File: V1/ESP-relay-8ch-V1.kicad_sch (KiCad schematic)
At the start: 142 parts, among them J1 +24VDC, J10 OUT1, J2 INPUTS, J3 OUT1, J4 OUT1, J5 OUT1, J6 OUT1, J7 OUT1, J8 OUT1, J9 OUT1, K1 G5PZ-1A, K2 G5PZ-1A, K3 G5PZ-1A, K4 G5PZ-1A, K5 G5PZ-1A, K6 G5PZ-1A, K7 G5PZ-1A, K8 G5PZ-1A, Q1 MMBT2222A/SOT-23-3, Q2 MMBT2222A/SOT-23-3, Q3 MMBT2222A/SOT-23-3, Q4 MMBT2222A/SOT-23-3, Q5 MMBT2222A/SOT-23-3, Q6 MMBT2222A/SOT-23-3, Q7 MMBT2222A/SOT-23-3, Q8 MMBT2222A/SOT-23-3, U1 SY8089A1AAC, U10 TX4138, U11 Olimex_ESP32-POE, U2 LTV-817S, U3 LTV-817S, U4 LTV-817S, U5 LTV-817S, U6 LTV-817S, U7 LTV-817S, U8 LTV-817S, U9 LTV-817S

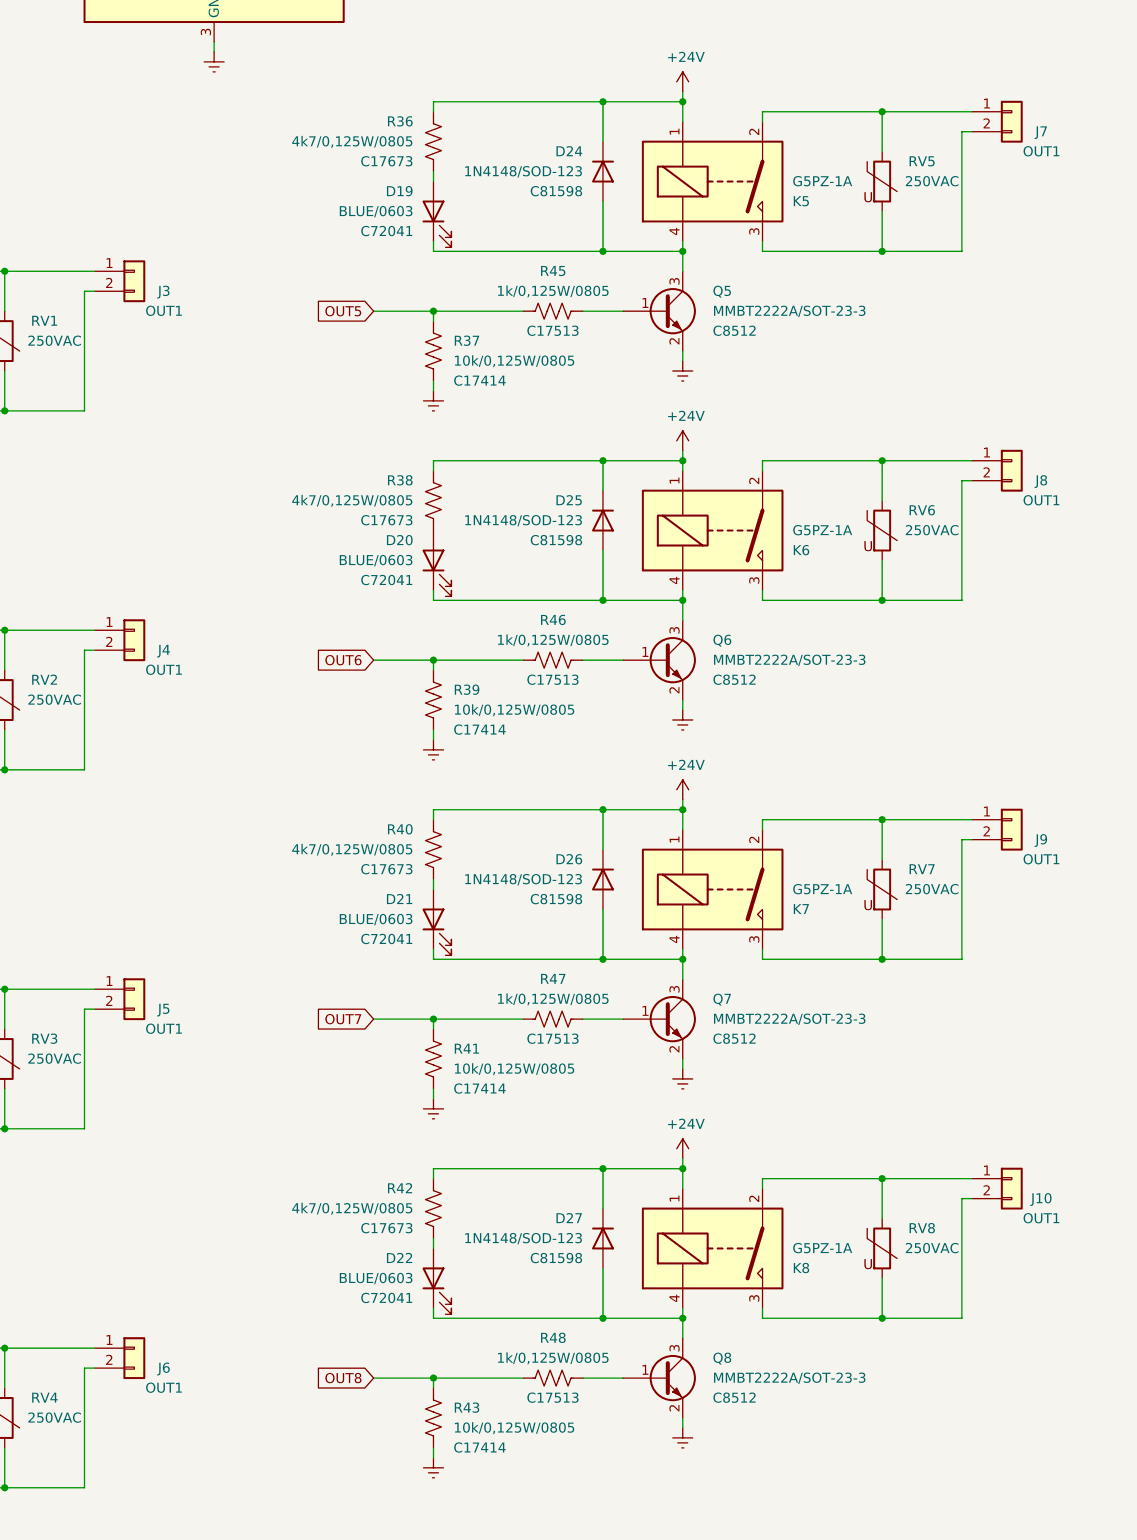
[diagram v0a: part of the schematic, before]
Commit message: Development
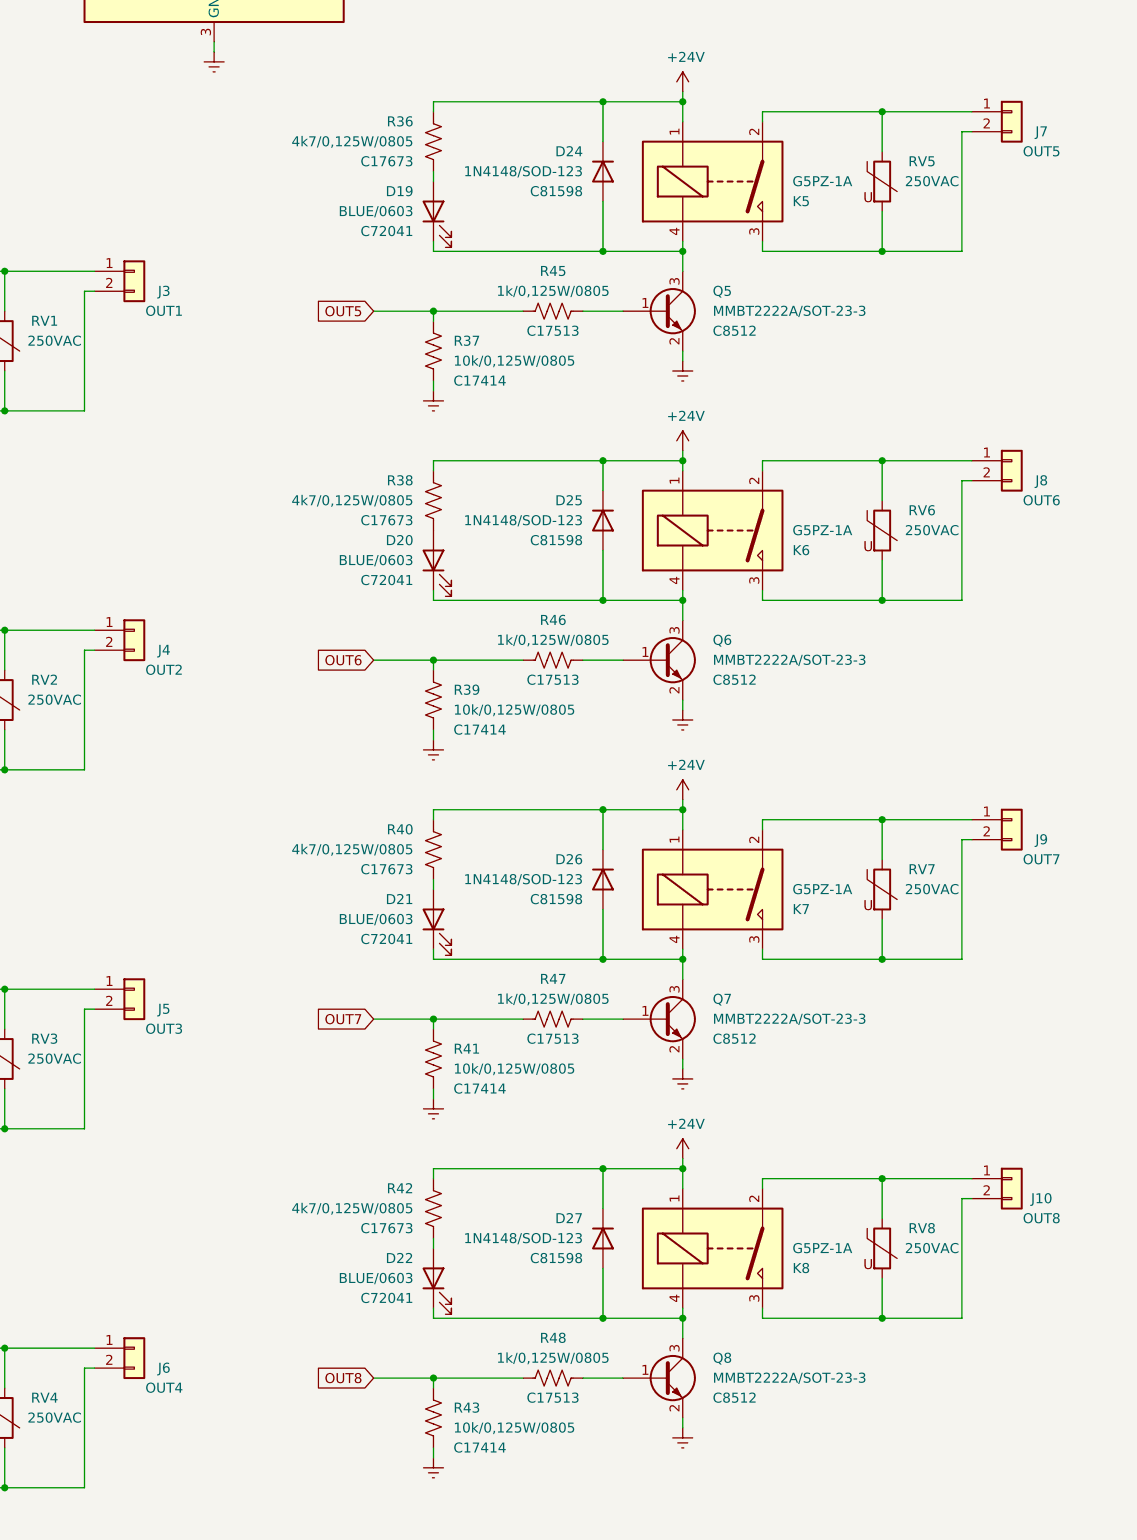
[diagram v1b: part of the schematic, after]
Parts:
- C1, C13: LCSC Part C1849 -> (none); LCSC Part # (none) -> C1849
- C10, C3, C4, C5, C6, C7, C8, C9: LCSC Part C1739 -> (none); LCSC Part # (none) -> C1739
- C11, C14: LCSC Part C49678 -> (none); LCSC Part # (none) -> C49678
- C12: LCSC Part C1653 -> (none); LCSC Part # (none) -> C1653
- C15: LCSC Part C38523 -> (none); LCSC Part # (none) -> C38523
- C16: LCSC Part C249930 -> (none); LCSC Part # (none) -> C249930
- C2: LCSC Part C263963 -> (none); LCSC Part # (none) -> C263963
- D1: LCSC Part C64898 -> (none); LCSC Part # (none) -> C64898
- D10: LCSC Part C65010 -> (none); LCSC Part # (none) -> C65010
- D11, D12, D13, D14, D19, D20, D21, D22: LCSC Part C72041 -> (none); LCSC Part # (none) -> C72041
- D15, D16, D17, D18, D24, D25, D26, D27: LCSC Part C81598 -> (none); LCSC Part # (none) -> C81598
- D2, D3, D4, D5, D6, D7, D8, D9: LCSC Part C109072 -> (none); LCSC Part # (none) -> C109072
- D23, D28, D29: LCSC Part C72043 -> (none); LCSC Part # (none) -> C72043
- J1: JLCPCB BOM (none) -> 0; Mfr (none) -> Metaltex; Mfr PN (none) -> BR902V; Vendor (none) -> Eletropeças; Vendor PN (none) -> 29273
- J10: value OUT1 -> OUT8
- J4: value OUT1 -> OUT2
- J5: value OUT1 -> OUT3
- J6: value OUT1 -> OUT4
- J7: value OUT1 -> OUT5
- J8: value OUT1 -> OUT6
- J9: value OUT1 -> OUT7
- L1: LCSC Part C370424 -> (none); LCSC Part # (none) -> C370424
- L2: LCSC Part C127788 -> (none); LCSC Part # (none) -> C127788
- Q1, Q2, Q3, Q4, Q5, Q6, Q7, Q8: LCSC Part C8512 -> (none); LCSC Part # (none) -> C8512
- R1, R2, R3, R4, R5, R6, R7, R8: LCSC Part C17379 -> (none); LCSC Part # (none) -> C17379
- R10: LCSC Part C149504 -> (none); LCSC Part # (none) -> C149504
- R11: LCSC Part C17552 -> (none); LCSC Part # (none) -> C17552
- R12, R13, R14, R15, R16, R17, R18, R19: LCSC Part C26010 -> (none); LCSC Part # (none) -> C26010
- R20: LCSC Part C17724 -> (none); LCSC Part # (none) -> C17724
- R21, R23, R25, R27, R35, R36, R38, R40, R42: LCSC Part C17673 -> (none); LCSC Part # (none) -> C17673
- R22, R24, R26, R28, R37, R39, R41, R43: LCSC Part C17414 -> (none); LCSC Part # (none) -> C17414
- R29: LCSC Part C17616 -> (none); LCSC Part # (none) -> C17616
- R30: LCSC Part C17758 -> (none); LCSC Part # (none) -> C17758
- R31, R32, R33, R34, R45, R46, R47, R48: LCSC Part C17513 -> (none); LCSC Part # (none) -> C17513
- R44: LCSC Part C4382 -> (none); LCSC Part # (none) -> C4382
- R49: LCSC Part C17837 -> (none); LCSC Part # (none) -> C17837
- R50: LCSC Part C17630 -> (none); LCSC Part # (none) -> C17630
- R9: LCSC Part C247605 -> (none); LCSC Part # (none) -> C247605
- U1: LCSC Part C479074 -> (none); LCSC Part # (none) -> C479074
- U10: LCSC Part C329267 -> (none); LCSC Part # (none) -> C329267
- U2, U3, U4, U5, U6, U7, U8, U9: LCSC Part C109227 -> (none); LCSC Part # (none) -> C109227
